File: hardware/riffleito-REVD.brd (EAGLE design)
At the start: 68.7 x 18 mm, 29 parts, among them IC1 ATMEGA328P, IC2 24AA128SN, IC4 MCP1700-33, X1 16 MHz

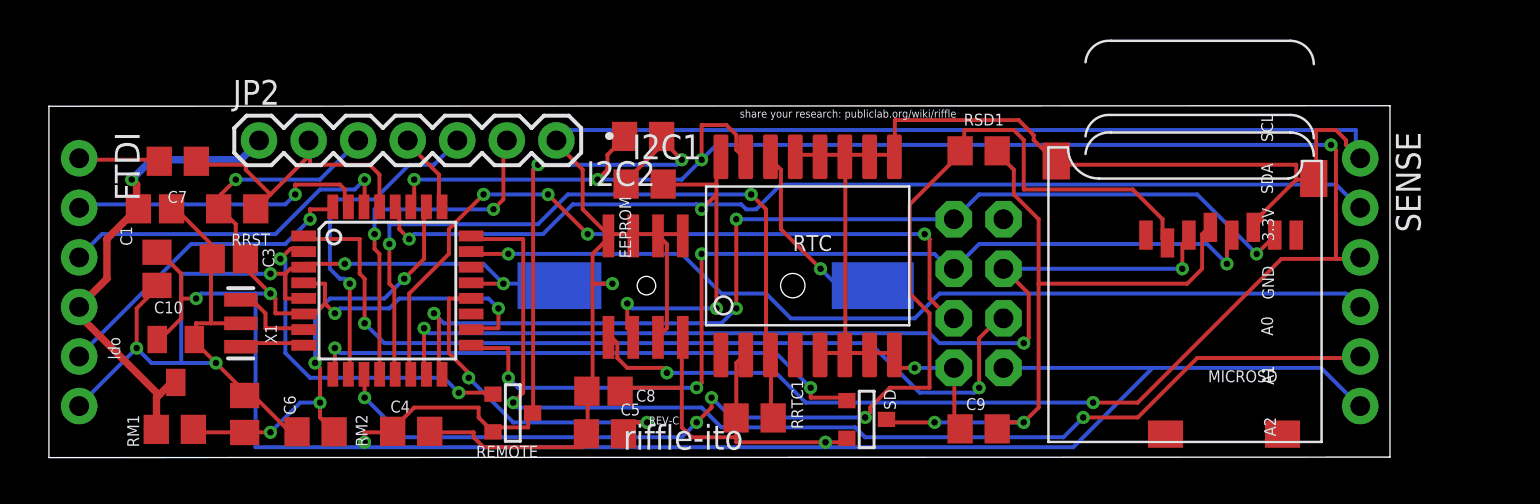
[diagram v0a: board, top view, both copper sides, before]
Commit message: update
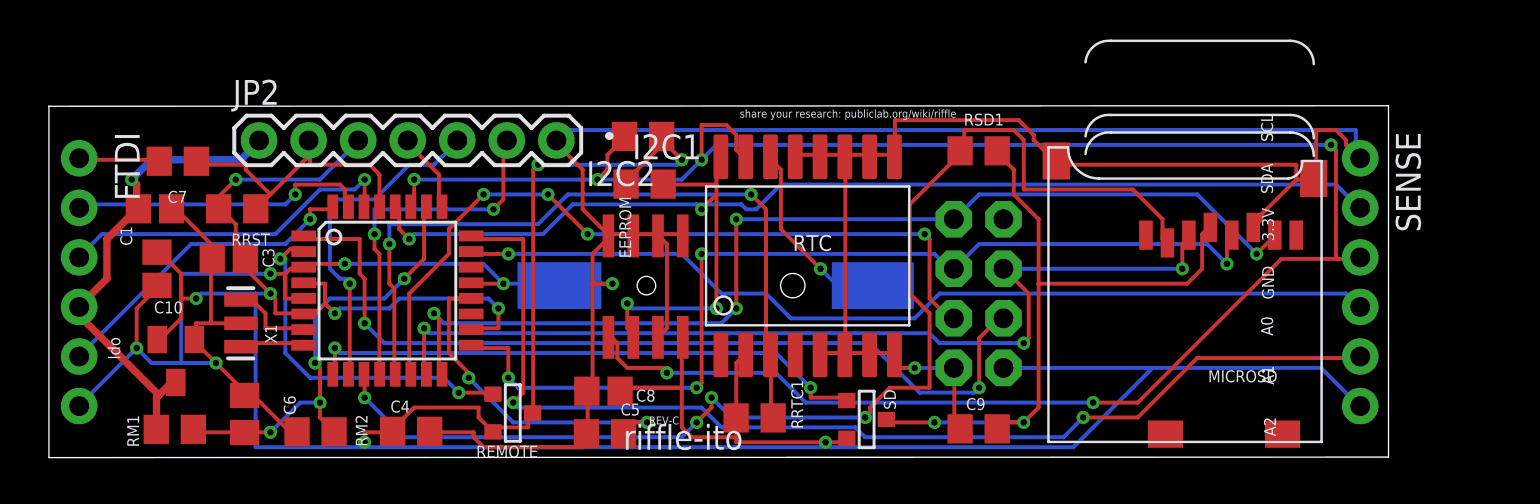
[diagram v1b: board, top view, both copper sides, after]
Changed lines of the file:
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@@
 <plain>
 <wire x1="0.5842" y1="-0.0254" x2="0.5842" y2="17.9832" width="0" layer="20"/>
-<wire x1="0.5842" y1="17.9832" x2="69.3166" y2="18.0086" width="0" layer="20"/>
-<wire x1="69.3166" y1="18.0086" x2="69.3166" y2="0" width="0" layer="20"/>
-<wire x1="69.3166" y1="0" x2="0.5842" y2="-0.0254" width="0" layer="20"/>
+<wire x1="0.5842" y1="17.9832" x2="69.2404" y2="18.0086" width="0" layer="20"/>
+<wire x1="69.2404" y1="18.0086" x2="69.2404" y2="0" width="0" layer="20"/>
+<wire x1="69.2404" y1="0" x2="0.5842" y2="-0.0254" width="0" layer="20"/>
 <text x="4.2418" y="5.0038" size="0.6096" layer="21" rot="R90">ldo</text>
 <text x="29.8196" y="13.3604" size="0.6096" layer="21" rot="R270">EEPROM</text>

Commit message: update
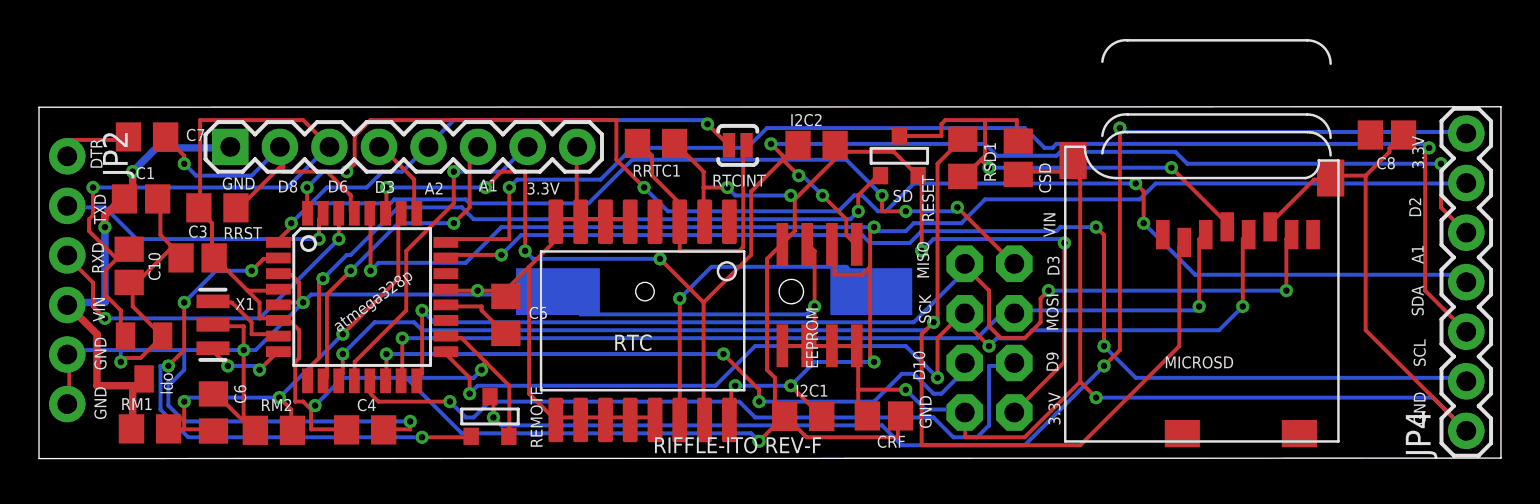
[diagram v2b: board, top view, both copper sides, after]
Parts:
- removed C9: .1uF, rcl:C0805@1
- removed FTDI, SENSE: (no value), SparkFun-Connectors:1X06
- removed RAD: M04X2, SparkFun-Connectors:2X4
- added CRF: 100u, resistor:C0805
- added CSD: .1uF, resistor:C0805
- added JP1: (no value), SparkFun-Connectors:1X08
- added JP4: (no value), SparkFun-Connectors:1X07
- added RTCINT: SOLDERJUMPERNO, _SparkFun:SJ_2S-NO
- added U$1: M04X2, SparkFun-Connectors:2X4
- JP2: device SparkFun-Connectors:1X07 -> SparkFun-Connectors:1X06
- moved C8 42.2 mm to (69.2, 16.5), turned to 180 degrees
- moved RRTC1 15.0 mm to (31.7, 16.1), turned to 180 degrees
- moved I2C1 14.4 mm to (39.2, 2.08)
- moved SD 13.6 mm to (44.2, 15.4), turned to 180 degrees
- moved JP2 9.86 mm to (1.52, 15.4), turned to 270 degrees
- moved RTC 9.09 mm to (31.0, 6.99), turned to 180 degrees
- moved IC2 8.93 mm to (40.1, 8.31), turned to 0 degrees
- moved I2C2 8.90 mm to (39.9, 16.0)
- moved C5 7.94 mm to (24.0, 7.29), turned to 270 degrees
- moved C4 2.36 mm to (16.8, 1.40)
- moved RM2 2.13 mm to (12.1, 1.37)
- moved C7 2.01 mm to (5.61, 16.4)
- moved IC4 1.64 mm to (5.46, 5.11)
- moved C6 1.60 mm to (9.02, 2.29)
- moved C3 1.60 mm to (8.20, 10.2)
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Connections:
- new net N$1: RRTC1.2, RTC.3, RTCINT.1
- new net N$4: JP4.7, REMOTE.1
- net A0: now also JP4.2; no longer SENSE.4
- net A1: now also JP4.3; no longer SENSE.5
- net A2: now also JP1.4; no longer JP2.4
- net D10: now also U$1.6; no longer RAD.3
- net D2: now also JP4.4; no longer FTDI.5
- net D3: now also JP1.5, RTCINT.2, U$1.1; no longer RAD.4
- net D6: now also JP1.6; no longer JP2.5
- net D8: now also JP1.7; no longer JP2.6
- net D9: now also U$1.5; no longer RRTC1.2, RTC.3
- net DTR: now also JP2.1; no longer FTDI.1
- net GND: now also CRF.2, CSD.2, JP1.8, JP2.5, JP2.6, JP4.1, U$1.8; no longer C9.1, FTDI.6, JP2.7, RAD.1, SENSE.1
- net MISO: now also U$1.2; no longer RAD.7
- net MOSI: now also U$1.3; no longer RAD.6
- net RESET: now also JP1.2; no longer JP2.2
- net RXD: now also JP2.3; no longer FTDI.3
- net SCK: now also U$1.4; no longer RAD.5
- net SCL: now also JP4.6; no longer SENSE.2
- net SDA: now also JP4.5; no longer SENSE.3
- net TXD: now also JP2.2; no longer FTDI.2
- net VCC: now also CRF.1, JP1.3, U$1.7; no longer C8.2, JP2.3, RAD.2, REMOTE.1, SENSE.6
- net VDD: now also CSD.1; no longer C9.2
- net VIN: now also JP1.1, JP2.4; no longer FTDI.4, JP2.1
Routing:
- net N$4: track 0.00 -> 65.2 mm, vias 0 -> 3
- net D2: track 16.5 -> 70.5 mm, vias 1 -> 5
- net VCC: track 176.2 -> 151.4 mm, vias 9 -> 8
- net D3: track 44.7 -> 66.4 mm, vias 2 -> 5
- net SDA: track 106.6 -> 85.3 mm, vias 6 -> 8
- net N$1: track 0.00 -> 15.1 mm
- net AREF: track 17.5 -> 3.89 mm, vias 2 -> 0
- net SCL: track 71.2 -> 83.5 mm, vias 4 -> 5
- net A0: track 47.8 -> 60.0 mm, vias 1 -> 3
- net D4: track 18.0 -> 28.5 mm, vias 2 -> 4
- net VDD: track 34.9 -> 25.4 mm
- net A1: track 57.2 -> 65.4 mm
- net D5: track 29.1 -> 37.3 mm
- net RTC_BATT: track 9.82 -> 17.2 mm
- net D7: track 63.1 -> 70.1 mm, vias 4 -> 2
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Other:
- board size 68.7 x 18 mm -> 74.9 x 18 mm
- board text added: "<<nordic RF24>>"
- board text added: "CERN OHL v1.2"
- board text added: "D10"
- board text added: "D3"
- board text added: "D9"
- board text added: "RIFFLE-IT REV-F"
- board text added: "RIFFLE-ITO REV-F"
- board text added: "atmega328p"
- board text added: "publicab.org/wiki/riffle"
- board text removed: "A0"
- board text removed: "CERN Open Hardware License Ver. 1.2"
- board text removed: "REV-C"
- board text removed: "riffle-ito"
- board text removed: "share your research: publiclab.org/wiki/riffle"
